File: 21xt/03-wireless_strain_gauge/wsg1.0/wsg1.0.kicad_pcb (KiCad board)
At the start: 2 copper layers, 34 parts, among them J1 GenConn3, J2 GenConn1, J3 GenConn2, U1 ADS1120, U2 102010388

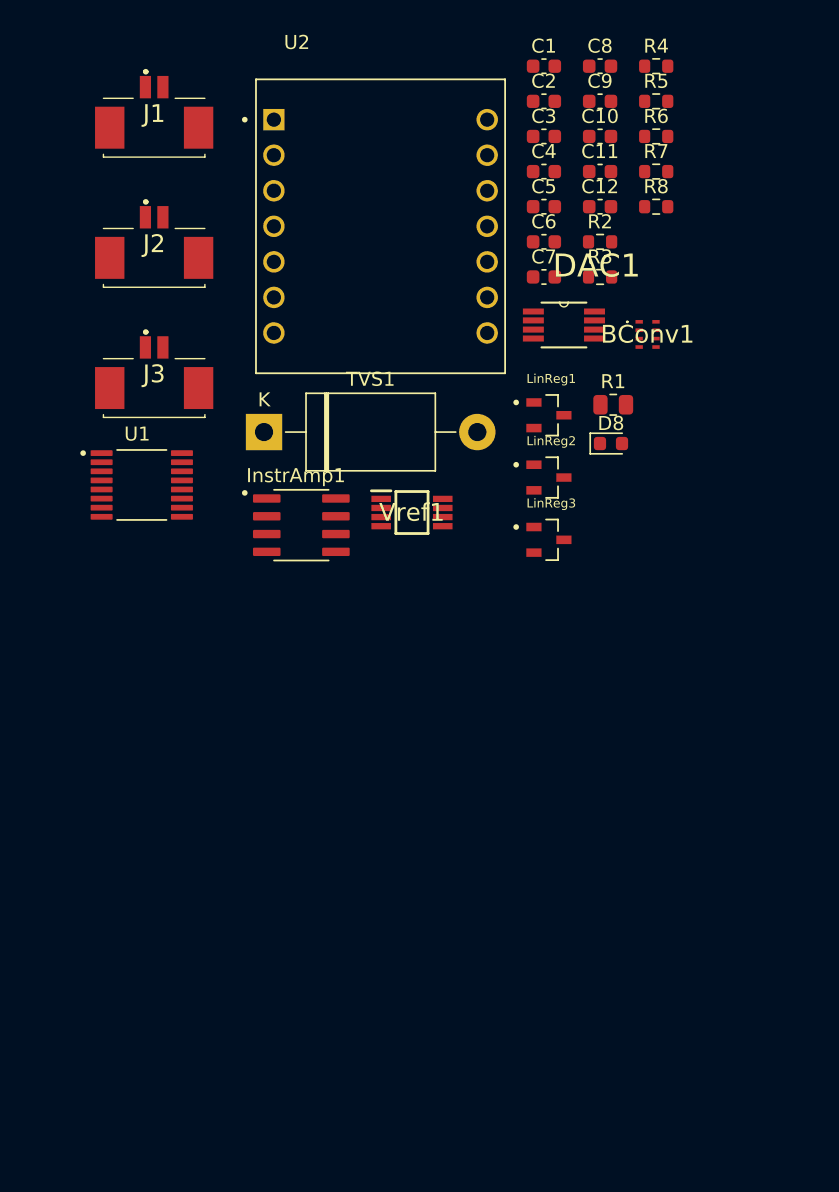
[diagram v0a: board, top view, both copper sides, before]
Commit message: First layout 'draft'
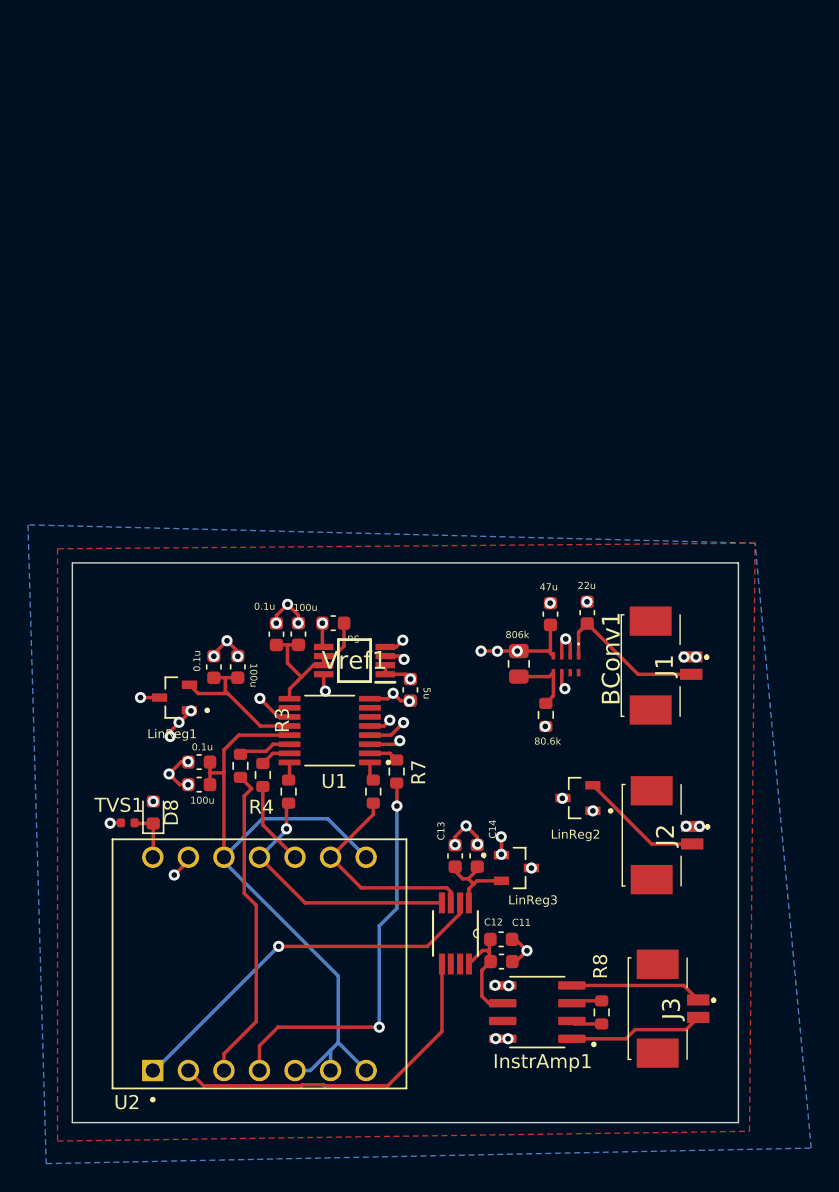
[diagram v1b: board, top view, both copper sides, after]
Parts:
- removed C1: 22uF, Capacitor_SMD:C_0603_1608Metric
- removed C2: 47uF, Capacitor_SMD:C_0603_1608Metric
- removed R1: 806k, Resistor_SMD:R_0805_2012Metric
- removed R2: 80.6k, Resistor_SMD:R_0603_1608Metric
- added 22u: 22uF, Capacitor_SMD:C_0603_1608Metric, F.Cu at (127.7, 102.7)
- added 47u: 47uF, Capacitor_SMD:C_0603_1608Metric, F.Cu at (125.1, 102.8)
- added 80.6k: 80.6k, Resistor_SMD:R_0603_1608Metric, F.Cu at (124.8, 110.0)
- added 806k: 806k, Resistor_SMD:R_0805_2012Metric, F.Cu at (122.8, 106.4)
- added C13: 0.1uF, Capacitor_SMD:C_0603_1608Metric, F.Cu at (118.3, 120.1)
- added C14: 100uF, Capacitor_SMD:C_0603_1608Metric, F.Cu at (119.9, 120.1)
- TVS1: footprint Diode_THT:D_DO-201AE_P15.24mm_Horizontal -> Diode_SMD:D_0402_1005Metric
- moved J3 58.5 mm to (133.8, 131.0), turned to -90 degrees
- moved R4 57.9 mm to (104.5, 114.3), turned to -90 degrees
- moved R8 57.7 mm to (128.8, 131.3), turned to 90 degrees
- moved J2 55.9 mm to (133.3, 118.6), turned to -90 degrees
- moved C11 55.3 mm to (121.6, 126.1)
- moved C12 54.4 mm to (121.6, 127.6)
- moved J1 53.7 mm to (133.2, 106.5), turned to -90 degrees
- moved R6 53.7 mm to (106.4, 115.5), turned to -90 degrees
- moved U2 53.4 mm to (104.3, 127.8), turned to 90 degrees
- moved R5 53.3 mm to (112.4, 115.5), turned to -90 degrees
- moved C3 52.5 mm to (100.0, 115.0), turned to 180 degrees
- moved C8 51.0 mm to (101.0, 106.6), turned to 90 degrees
- moved C4 48.9 mm to (100.0, 113.4), turned to 180 degrees
- moved R7 46.7 mm to (114.1, 114.1), turned to -90 degrees
- moved C9 44.5 mm to (105.5, 104.2), turned to 90 degrees
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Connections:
- DAC1 pad 2: CS -> CS-DAC
- DAC1 pad 6: DacClr -> unconnected-(DAC1-CLR#-Pad6)
- R7 pad 2: CS -> CS-ADC
- U2 pad 1: DacClr -> CS-DAC
- U2 pad 4: CS -> CS-ADC
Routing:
- net 3v3: track 0.00 -> 52.7 mm
- net CS-ADC: track 0.00 -> 28.8 mm, vias 0 -> 2
- net CS-DAC: track 0.00 -> 27.4 mm, vias 0 -> 1
- net DacLoad: track 0.00 -> 25.1 mm
- net GND: track 0.00 -> 24.3 mm, vias 0 -> 27
- net Ready: track 0.00 -> 22.8 mm
- net GND1: track 0.00 -> 20.4 mm, vias 0 -> 15
- net MOSI: track 0.00 -> 19.6 mm, vias 0 -> 1
- net SClk: track 0.00 -> 15.5 mm
- net Net-(U1-REFP0): track 0.00 -> 12.2 mm
- net 5.5V: track 0.00 -> 11.6 mm, vias 0 -> 10
- net Net-(BConv1-VIN): track 0.00 -> 11.5 mm
- net Net-(LinReg1-VOUT): track 0.00 -> 11.3 mm
- net Net-(InstrAmp1--IN): track 0.00 -> 9.66 mm
- net Net-(InstrAmp1-+IN): track 0.00 -> 9.46 mm
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- added copper zone on In1.Cu, net 5.5V
- added copper zone on F.Cu, net GND
- added copper zone on B.Cu, net GND1
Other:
- board outline added: 47.6 x 40 mm
- copper layers 2 -> 4
- board text added: "0.1u"
- board text added: "100u"
- board text added: "5u"
